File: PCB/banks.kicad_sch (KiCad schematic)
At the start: 50 parts, among them U1 XC7A50T-FGG484, Y3 100MHz

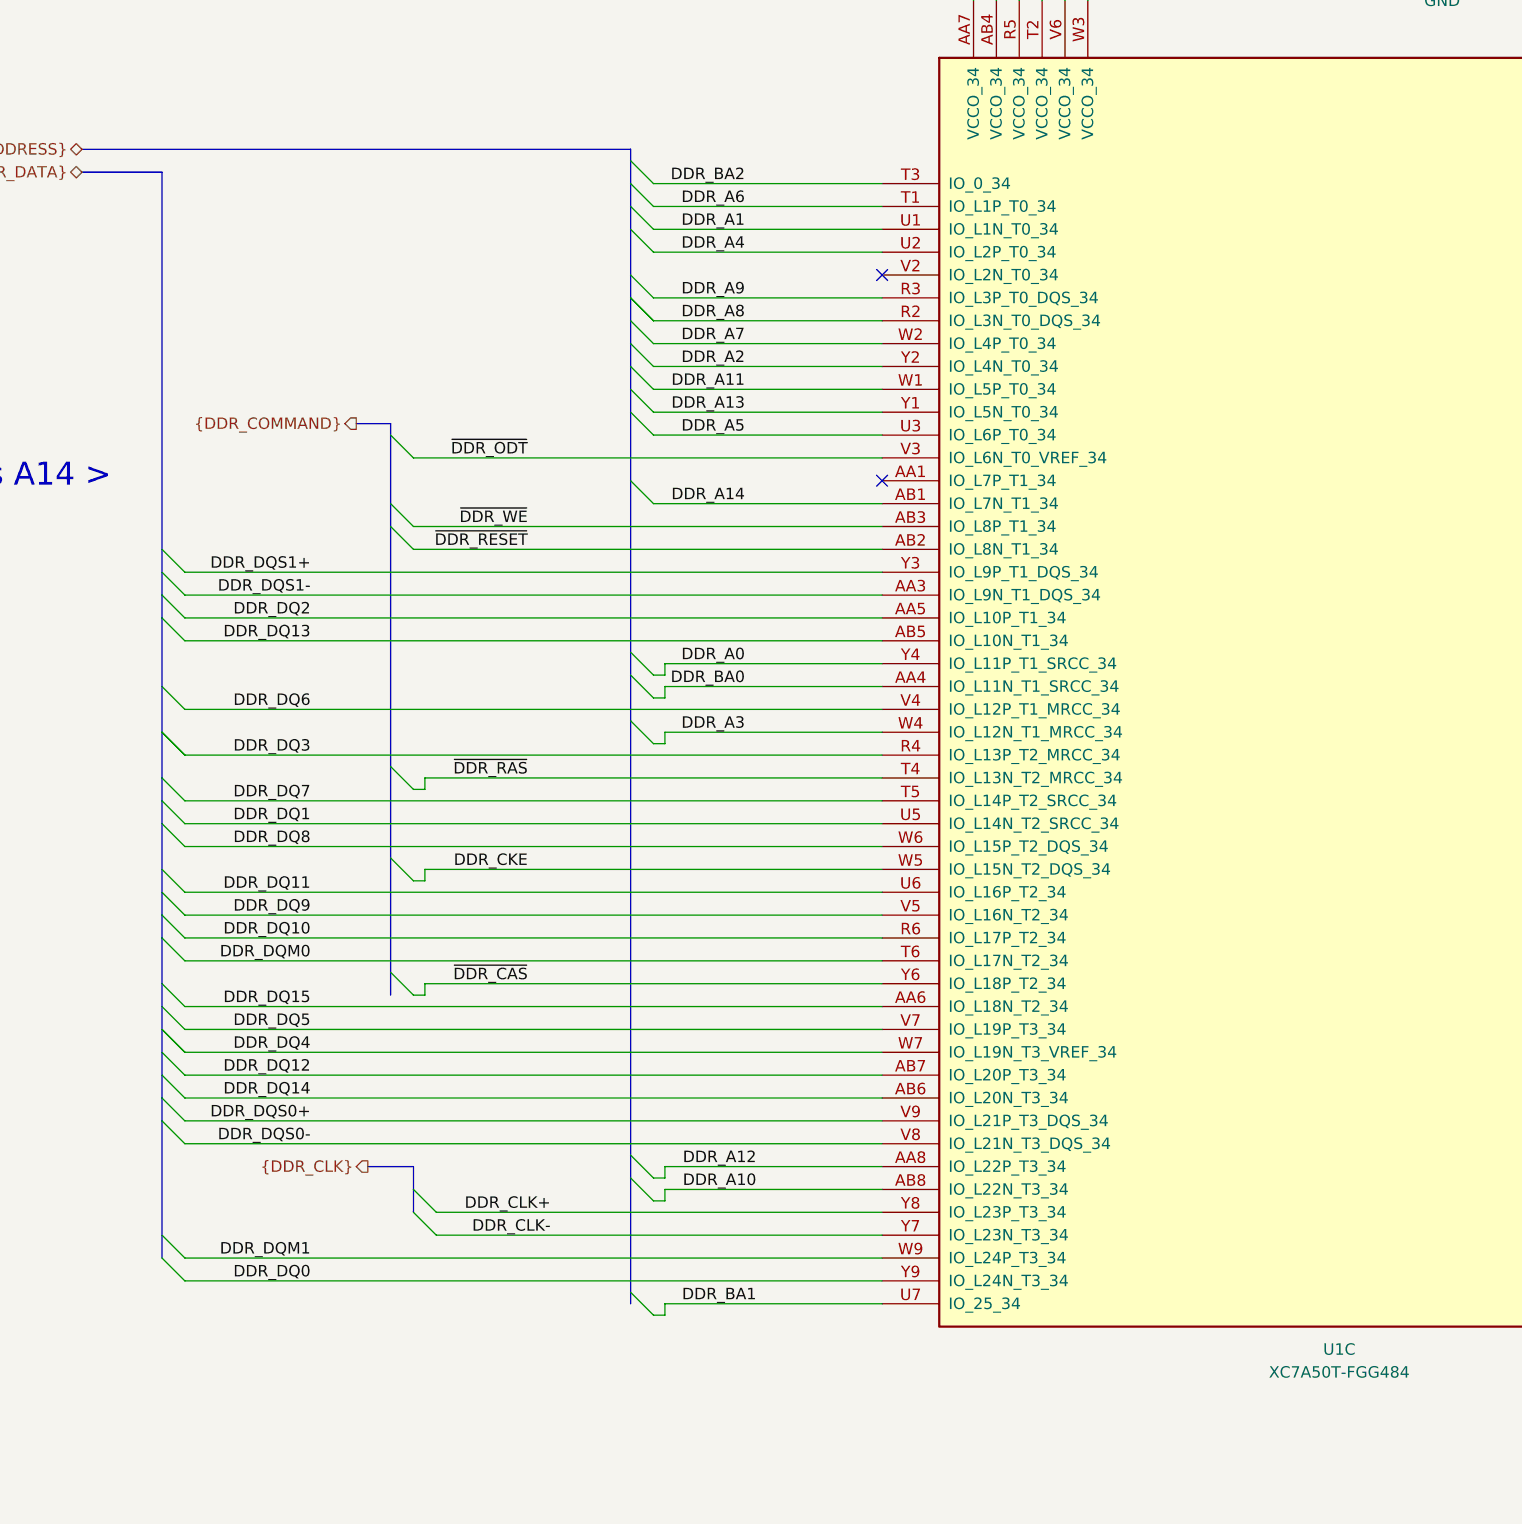
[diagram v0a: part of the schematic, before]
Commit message: a bunch of wiring
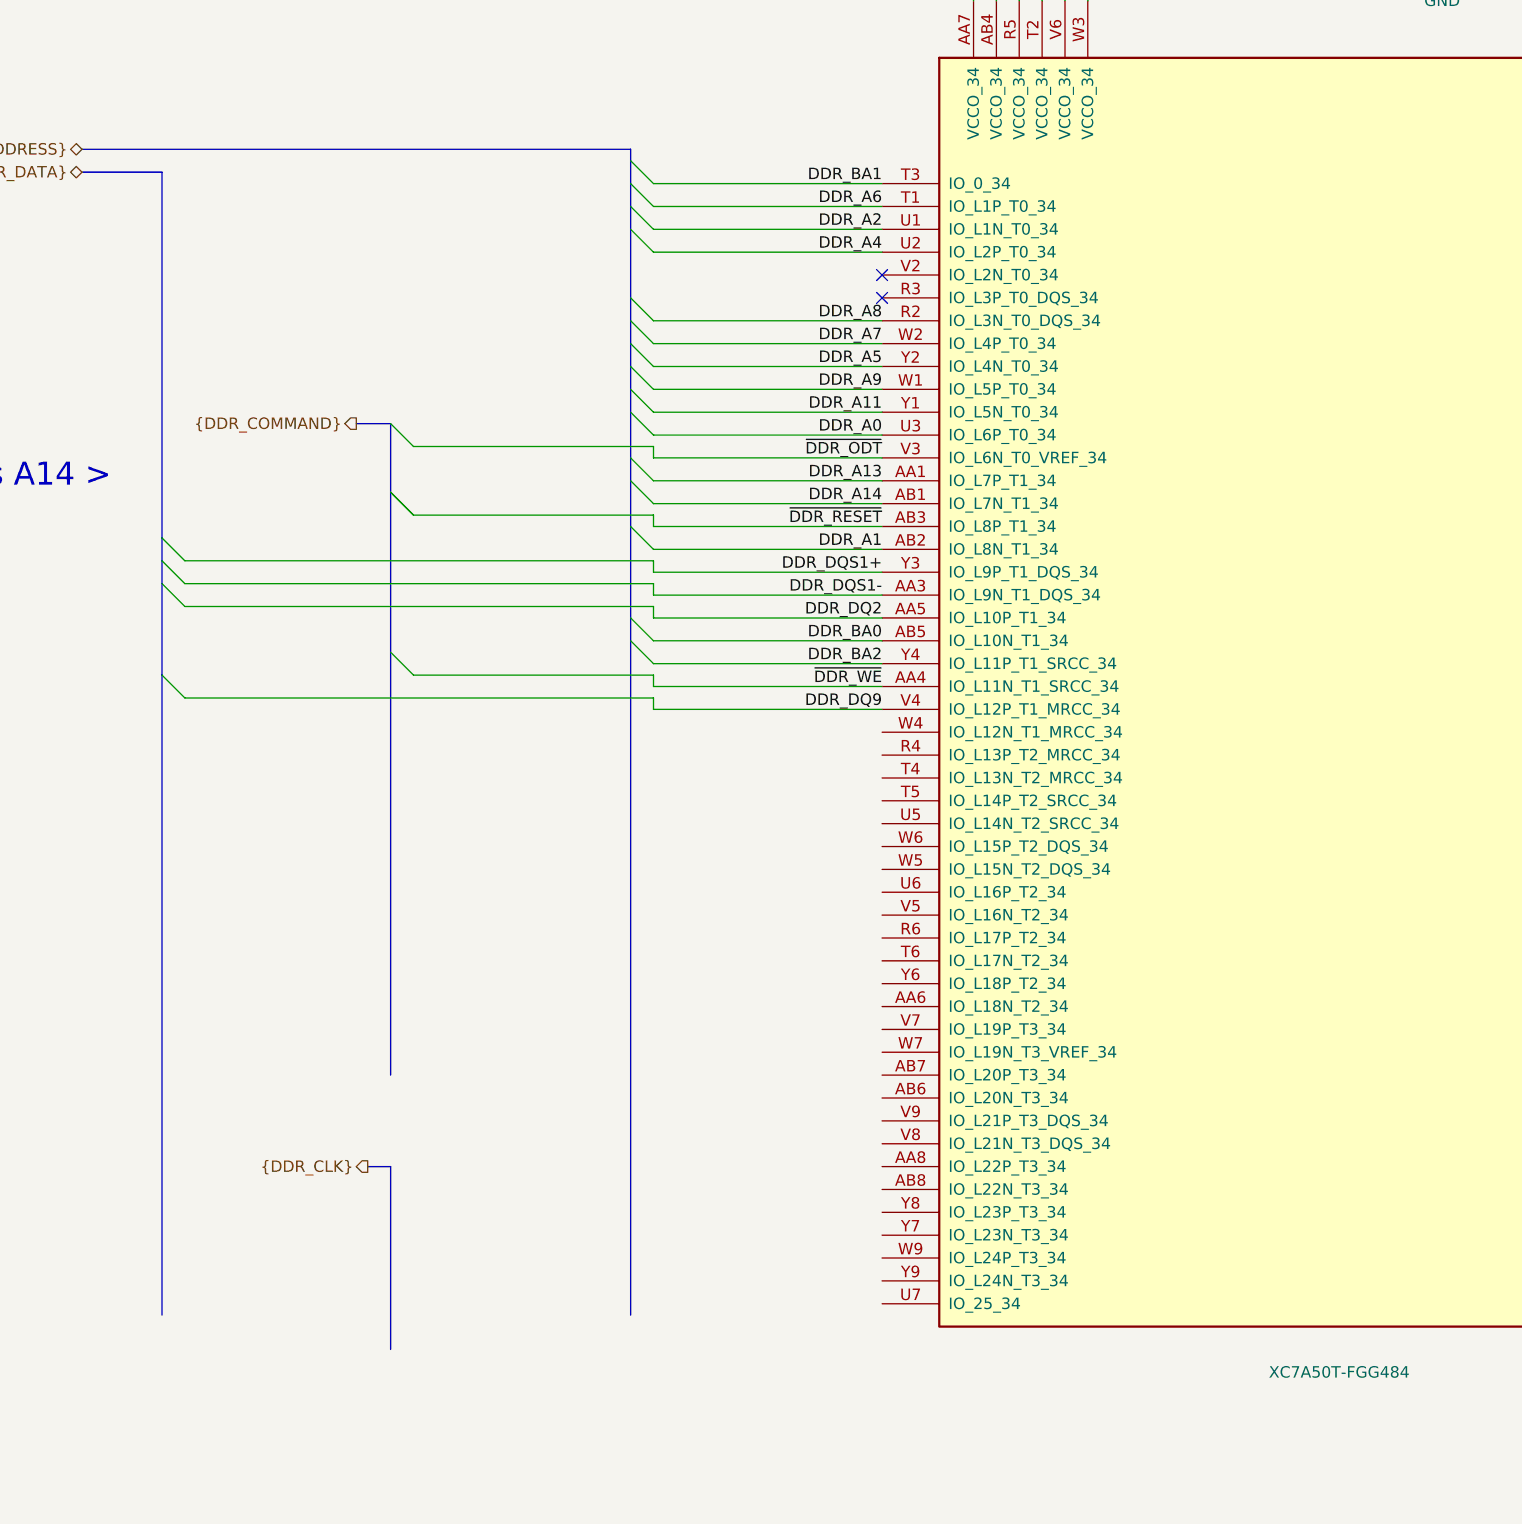
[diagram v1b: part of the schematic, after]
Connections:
- net DDR_DQ13 is gone; now on net DDR_BA0: U1.AB5 (IO_L10N_T1_34)
- net DDR_DQ6 is gone; now on net DDR_DQ9: U1.V4 (IO_L12P_T1_MRCC_34)
- net DDR_A0: now also U1.U3 (IO_L6P_T0_34); no longer U1.Y4 (IO_L11P_T1_SRCC_34)
- net DDR_A1: now also U1.AB2 (IO_L8N_T1_34); no longer U1.U1 (IO_L1N_T0_34)
- net DDR_A11: now also U1.Y1 (IO_L5N_T0_34); no longer U1.W1 (IO_L5P_T0_34)
- net DDR_A13: now also U1.AA1 (IO_L7P_T1_34); no longer U1.Y1 (IO_L5N_T0_34)
- net DDR_A2: now also U1.U1 (IO_L1N_T0_34); no longer U1.Y2 (IO_L4N_T0_34)
- net DDR_A5: now also U1.Y2 (IO_L4N_T0_34); no longer U1.U3 (IO_L6P_T0_34)
- net DDR_A9: now also U1.W1 (IO_L5P_T0_34); no longer U1.R3 (IO_L3P_T0_DQS_34)
- net DDR_BA0: no longer U1.AA4 (IO_L11N_T1_SRCC_34)
- net DDR_BA1: now also U1.T3 (IO_0_34); no longer U1.U7 (IO_25_34)
- net DDR_BA2: now also U1.Y4 (IO_L11P_T1_SRCC_34); no longer U1.T3 (IO_0_34)
- net DDR_DQ9: no longer U1.V5 (IO_L16N_T2_34)
- net ~{DDR_RESET}: now also U1.AB3 (IO_L8P_T1_34); no longer U1.AB2 (IO_L8N_T1_34)
- net ~{DDR_WE}: now also U1.AA4 (IO_L11N_T1_SRCC_34); no longer U1.AB3 (IO_L8P_T1_34)
- net DDR_A10: no longer names the net of U1.AB8 (IO_L22N_T3_34)
- net DDR_A12: no longer names the net of U1.AA8 (IO_L22P_T3_34)
- net DDR_A3: no longer names the net of U1.W4 (IO_L12N_T1_MRCC_34)
- net DDR_CKE: no longer names the net of U1.W5 (IO_L15N_T2_DQS_34)
- net DDR_CLK+: no longer names the net of U1.Y8 (IO_L23P_T3_34)
- net DDR_CLK-: no longer names the net of U1.Y7 (IO_L23N_T3_34)
- net DDR_DQ0: no longer names the net of U1.Y9 (IO_L24N_T3_34)
- net DDR_DQ1: no longer names the net of U1.U5 (IO_L14N_T2_SRCC_34)
- net DDR_DQ10: no longer names the net of U1.R6 (IO_L17P_T2_34)
- net DDR_DQ11: no longer names the net of U1.U6 (IO_L16P_T2_34)
- net DDR_DQ12: no longer names the net of U1.AB7 (IO_L20P_T3_34)
- net DDR_DQ14: no longer names the net of U1.AB6 (IO_L20N_T3_34)
- net DDR_DQ15: no longer names the net of U1.AA6 (IO_L18N_T2_34)
- net DDR_DQ3: no longer names the net of U1.R4 (IO_L13P_T2_MRCC_34)
- net DDR_DQ4: no longer names the net of U1.W7 (IO_L19N_T3_VREF_34)
- net DDR_DQ5: no longer names the net of U1.V7 (IO_L19P_T3_34)
- net DDR_DQ7: no longer names the net of U1.T5 (IO_L14P_T2_SRCC_34)
- net DDR_DQ8: no longer names the net of U1.W6 (IO_L15P_T2_DQS_34)
- net DDR_DQM0: no longer names the net of U1.T6 (IO_L17N_T2_34)
- net DDR_DQM1: no longer names the net of U1.W9 (IO_L24P_T3_34)
- net DDR_DQS0+: no longer names the net of U1.V9 (IO_L21P_T3_DQS_34)
- net DDR_DQS0-: no longer names the net of U1.V8 (IO_L21N_T3_DQS_34)
- net ~{DDR_CAS}: no longer names the net of U1.Y6 (IO_L18P_T2_34)
- net ~{DDR_RAS}: no longer names the net of U1.T4 (IO_L13N_T2_MRCC_34)

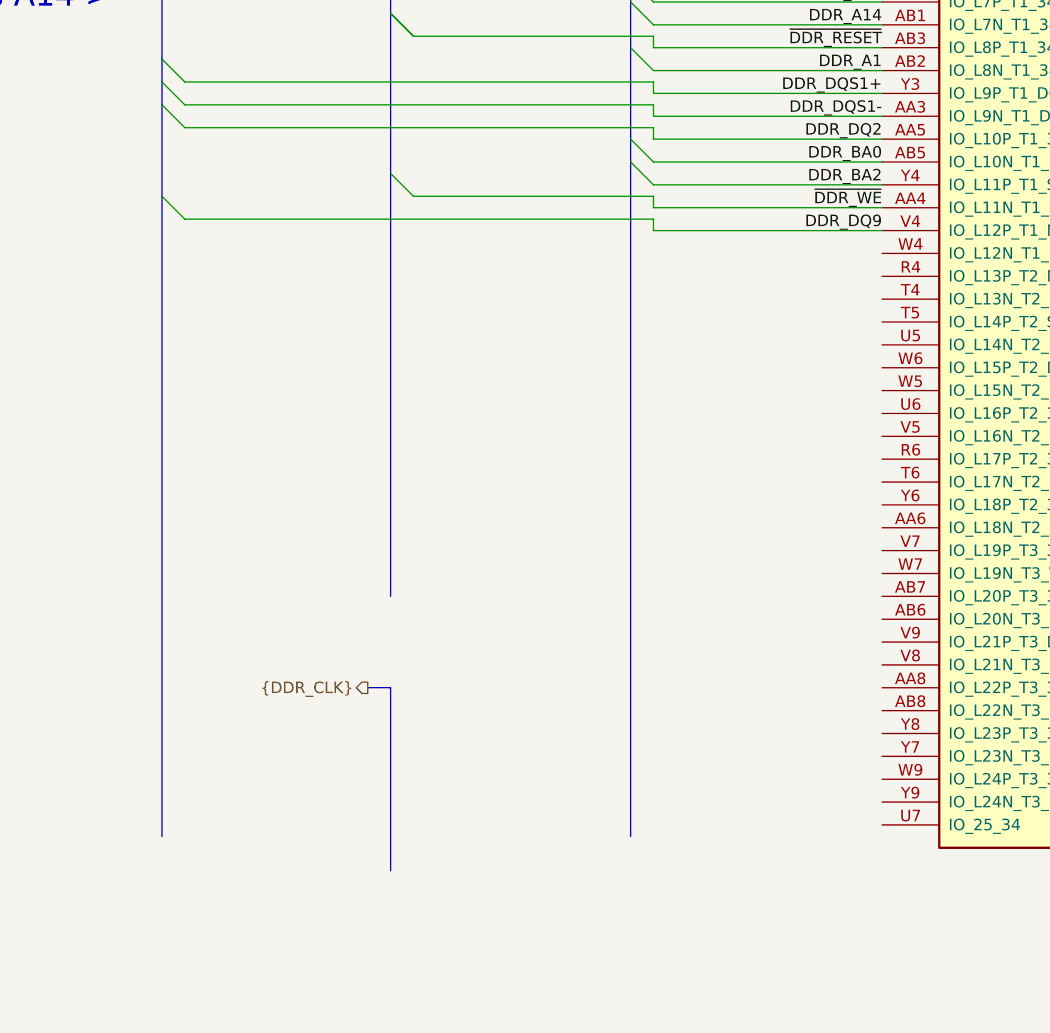
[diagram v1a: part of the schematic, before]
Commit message: finished wiring
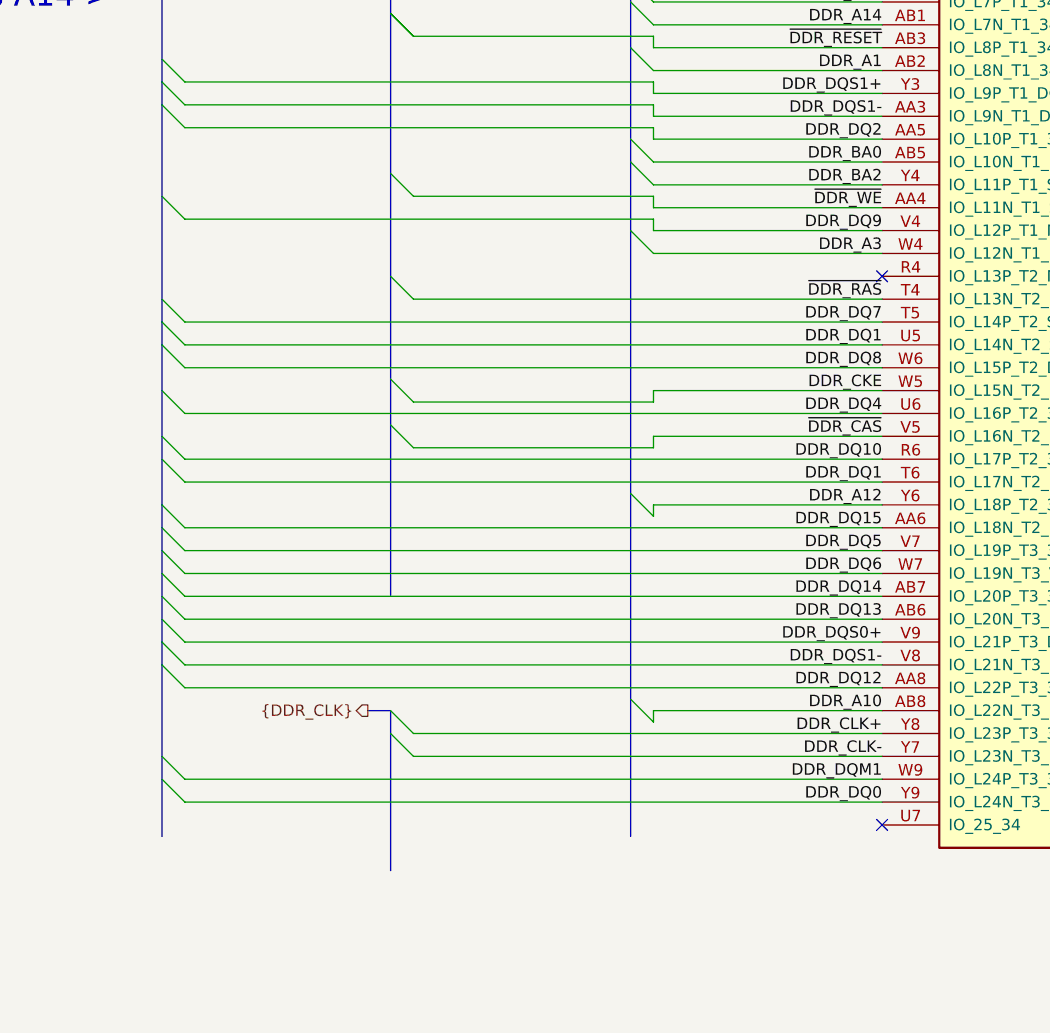
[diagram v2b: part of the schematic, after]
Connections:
- net DDR_DQS1-: now also U1.V8 (IO_L21N_T3_DQS_34)
- net DDR_DQ15: now reaches U1.AA6 (IO_L18N_T2_34)
- net DDR_DQ12: now reaches U1.AA8 (IO_L22P_T3_34)
- net DDR_DQ13: now reaches U1.AB6 (IO_L20N_T3_34)
- net DDR_DQ14: now reaches U1.AB7 (IO_L20P_T3_34)
- net DDR_A10: now reaches U1.AB8 (IO_L22N_T3_34)
- net DDR_DQ10: now reaches U1.R6 (IO_L17P_T2_34)
- net ~{DDR_RAS}: now reaches U1.T4 (IO_L13N_T2_MRCC_34)
- net DDR_DQ7: now reaches U1.T5 (IO_L14P_T2_SRCC_34)
- net DDR_DQ1: now reaches U1.T6 (IO_L17N_T2_34)
- net DDR_DQ1: now also U1.U5 (IO_L14N_T2_SRCC_34)
- net DDR_DQ4: now reaches U1.U6 (IO_L16P_T2_34)
- net ~{DDR_CAS}: now reaches U1.V5 (IO_L16N_T2_34)
- net DDR_DQ5: now reaches U1.V7 (IO_L19P_T3_34)
- net DDR_DQS0+: now reaches U1.V9 (IO_L21P_T3_DQS_34)
- net DDR_A3: now reaches U1.W4 (IO_L12N_T1_MRCC_34)
- net DDR_CKE: now reaches U1.W5 (IO_L15N_T2_DQS_34)
- net DDR_DQ8: now reaches U1.W6 (IO_L15P_T2_DQS_34)
- net DDR_DQ6: now reaches U1.W7 (IO_L19N_T3_VREF_34)
- net DDR_DQM1: now reaches U1.W9 (IO_L24P_T3_34)
- net DDR_A12: now reaches U1.Y6 (IO_L18P_T2_34)
- net DDR_CLK-: now reaches U1.Y7 (IO_L23N_T3_34)
- net DDR_CLK+: now reaches U1.Y8 (IO_L23P_T3_34)
- net DDR_DQ0: now reaches U1.Y9 (IO_L24N_T3_34)
- no-connect marks 12 -> 14
